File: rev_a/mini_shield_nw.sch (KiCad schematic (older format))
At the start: 3 parts

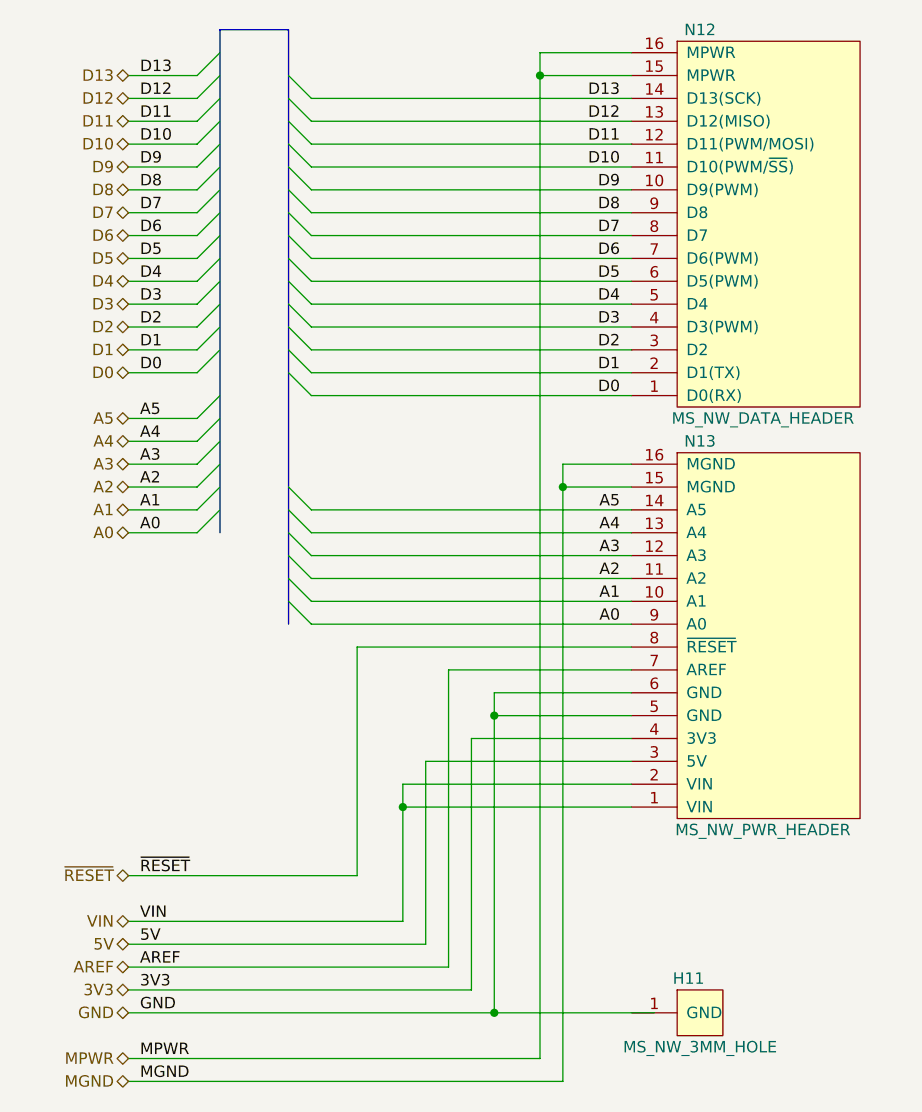
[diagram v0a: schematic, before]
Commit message: Rev. A of the Busino board layout is in pretty good shape.
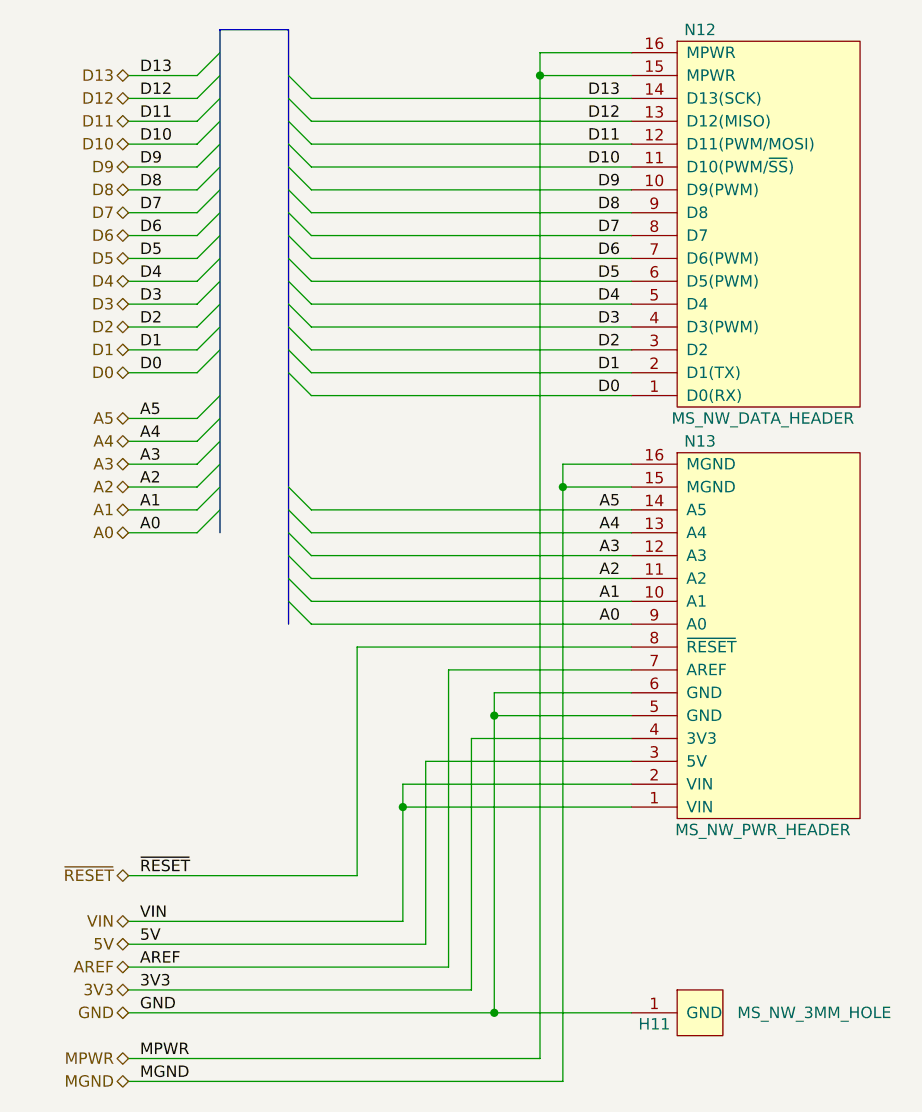
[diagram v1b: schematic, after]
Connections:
- net GND: now also H11.1 (GND)
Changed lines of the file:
@@
 LIBS:contrib
 LIBS:valves
-LIBS:mbino
 LIBS:busino-cache
 EELAYER 24 0
@@
 encoding utf-8
 Sheet 6 7
-Title ""
-Date ""
-Rev ""
+Title "Busino: North West Mini-Shield Connections"
+Date "08 Jul 2014"
+Rev "Rev. A"
 Comp ""
 Comment1 ""
@@
 	5400 5500 3900 5500
 Wire Wire Line
-	3900 5600 6200 5600
+	3900 5600 6100 5600
 Wire Wire Line
 	5700 5800 3900 5800
@@
 U 1 1 5396AEE1
 P 6400 5600
-F 0 "H11" H 6350 5750 50  0000 C CNN
-F 1 "MS_NW_3MM_HOLE" H 6400 5450 50  0000 C CNN
+F 0 "H11" H 6200 5550 50  0000 C CNN
+F 1 "MS_NW_3MM_HOLE" H 6900 5600 50  0000 C CNN
 F 2 "" H 6400 5600 60  0000 C CNN
 F 3 "" H 6400 5600 60  0000 C CNN
@@
 	4600 3800 4700 3900
 Wire Bus Line
-	4600 3900 4600 1300
+	4600 1300 4600 3900
 $EndSCHEMATC
